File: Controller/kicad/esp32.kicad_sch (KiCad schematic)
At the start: 9 parts, among them J11 PROG, J12 PI, SW1 RESET, SW2 BOOT, U4 ESP32-WROOM-32D

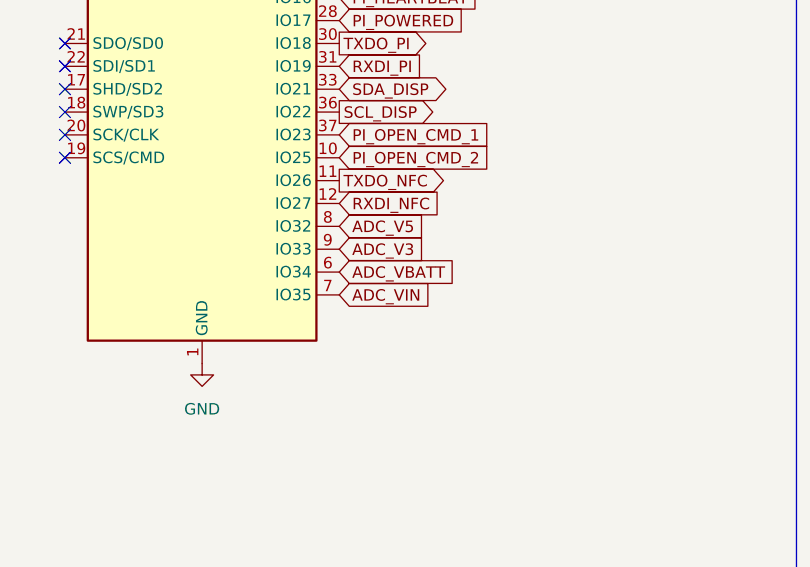
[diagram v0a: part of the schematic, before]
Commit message: Pre-production check-in
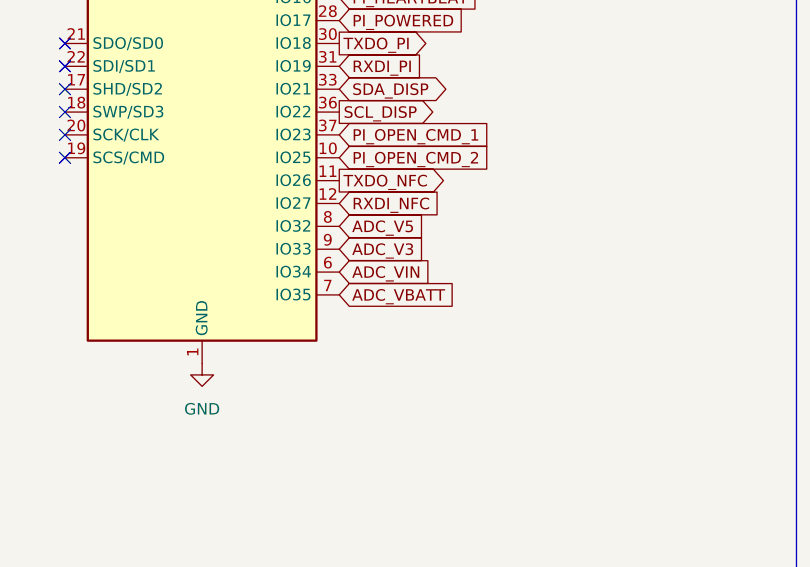
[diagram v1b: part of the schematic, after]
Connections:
- net ADC_VBATT: now also U4.7 (IO35); no longer U4.6 (IO34)
- net ADC_VIN: now also U4.6 (IO34); no longer U4.7 (IO35)
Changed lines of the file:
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@@
     )
   )
-  (global_label "ADC_VIN" (shape input) (at 223.52 121.92 0) (fields_autoplaced)
-    (effects (font (size 1.27 1.27)) (justify left))
-    (property "Intersheet References" "${INTERSHEET_REFS}" (id 0) (at 233.5531 121.8406 0)
+  (global_label "ADC_VIN" (shape input) (at 223.52 119.38 0) (fields_autoplaced)
+    (effects (font (size 1.27 1.27)) (justify left))
+    (property "Intersheet References" "${INTERSHEET_REFS}" (id 0) (at 233.5531 119.3006 0)
       (effects (font (size 1.27 1.27)) (justify left) hide)
     )
@@
     )
   )
-  (global_label "ADC_VBATT" (shape input) (at 223.52 119.38 0) (fields_autoplaced)
-    (effects (font (size 1.27 1.27)) (justify left))
-    (property "Intersheet References" "${INTERSHEET_REFS}" (id 0) (at 235.9117 119.3006 0)
+  (global_label "ADC_VBATT" (shape input) (at 223.52 121.92 0) (fields_autoplaced)
+    (effects (font (size 1.27 1.27)) (justify left))
+    (property "Intersheet References" "${INTERSHEET_REFS}" (id 0) (at 235.9117 121.8406 0)
       (effects (font (size 1.27 1.27)) (justify left) hide)
     )
@@
       (effects (font (size 1.27 1.27)) hide)
     )
-    (property "Datasheet" "https://datasheet.lcsc.com/lcsc/2002271431_XKB-Connectivity-TS-1187A-B-A-B_C318884.pdf" (id 3) (at 252.73 68.58 0)
+    (property "Datasheet" "~" (id 3) (at 252.73 68.58 0)
       (effects (font (size 1.27 1.27)) hide)
     )
@@
       (effects (font (size 1.27 1.27)) hide)
     )
-    (property "Datasheet" "https://datasheet.lcsc.com/lcsc/2002271431_XKB-Connectivity-TS-1187A-B-A-B_C318884.pdf" (id 3) (at 158.75 68.58 0)
+    (property "Datasheet" "~" (id 3) (at 158.75 68.58 0)
       (effects (font (size 1.27 1.27)) hide)
     )
@@
       (effects (font (size 1.27 1.27)) hide)
     )
-    (property "Datasheet" "https://datasheet.lcsc.com/lcsc/2110100730_XKB-Connectivity-X9555WV-2x04-6TV01_C2884546.pdf" (id 3) (at 67.31 165.1 0)
-      (effects (font (size 1.27 1.27)) hide)
-    )
+    (property "Datasheet" "~" (id 3) (at 67.31 165.1 0)
+      (effects (font (size 1.27 1.27)) hide)
+    )
